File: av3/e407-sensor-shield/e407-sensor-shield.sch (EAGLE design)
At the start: 26 parts, among them CON1 CON1, CON2 CON1, CON4 CON4, J1 ROCKETBUS

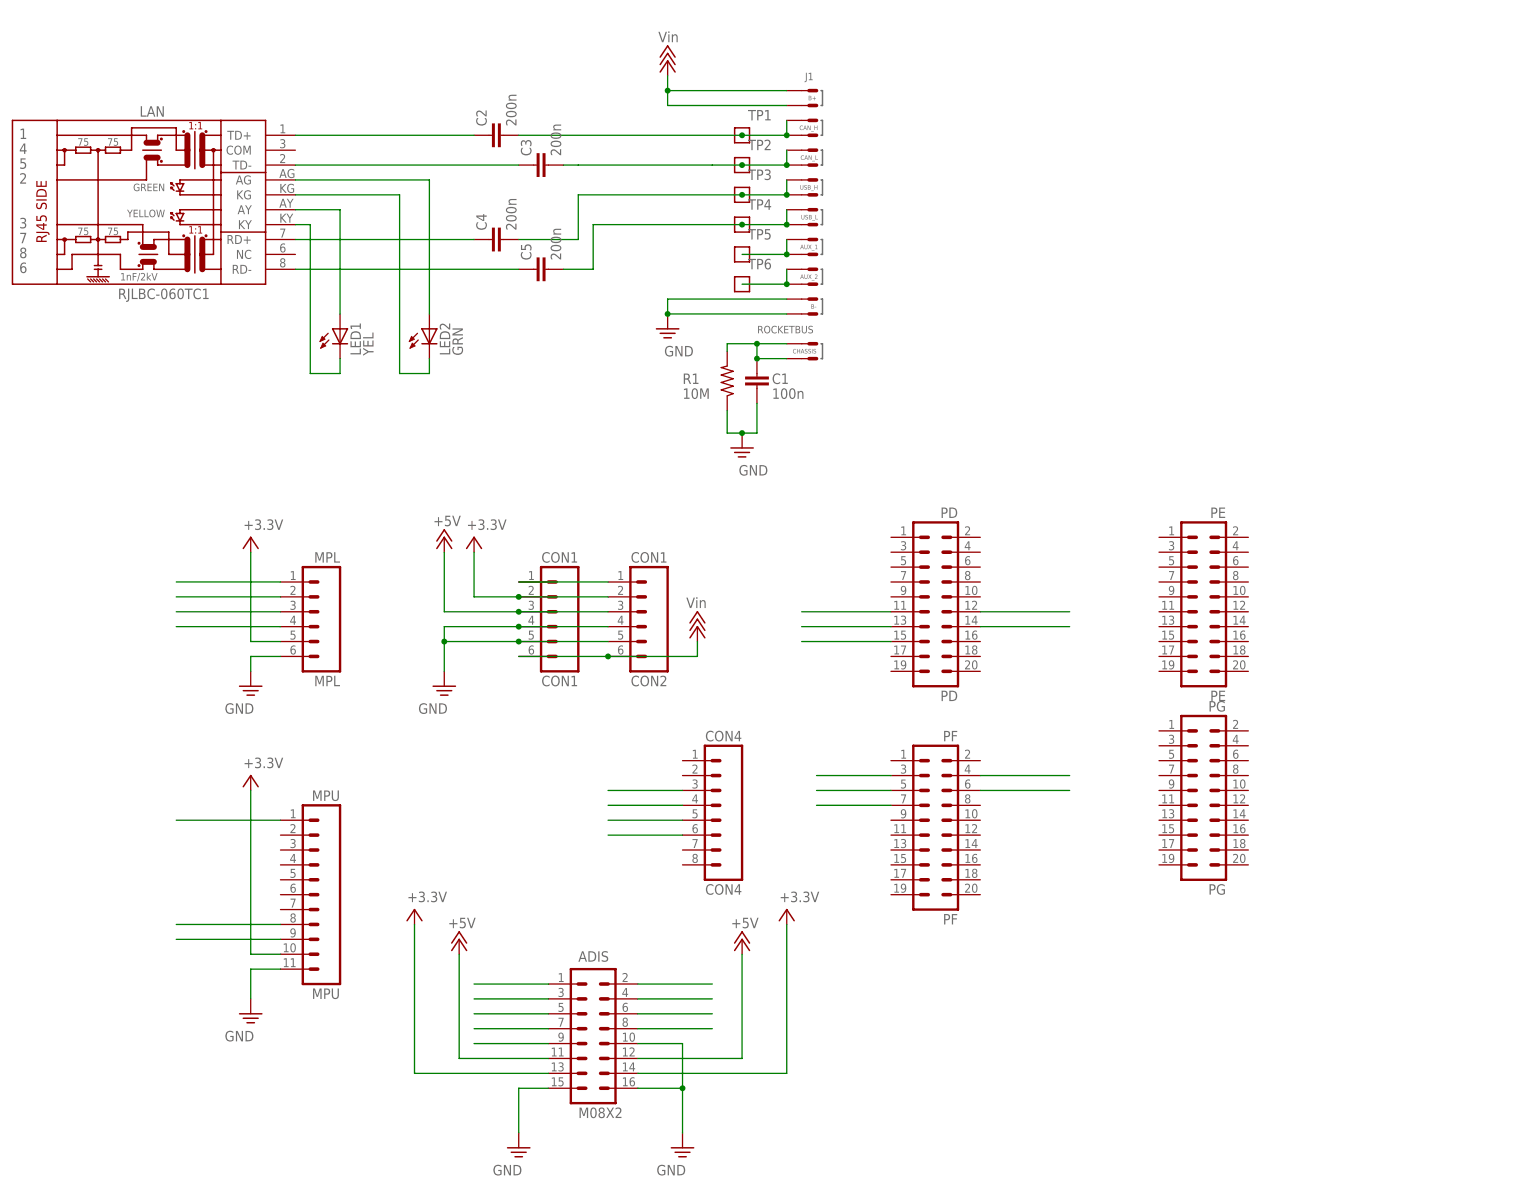
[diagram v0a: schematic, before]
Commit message: Added stupid EAGLE temporary files to the gitignore. Updated IMU adapter with sane net names so we could easily trace nets. And updated the e407 shield to add a RGB LED, correct some schematic mistakes found out while double checking connections, and updated to being routable on a PCB router.
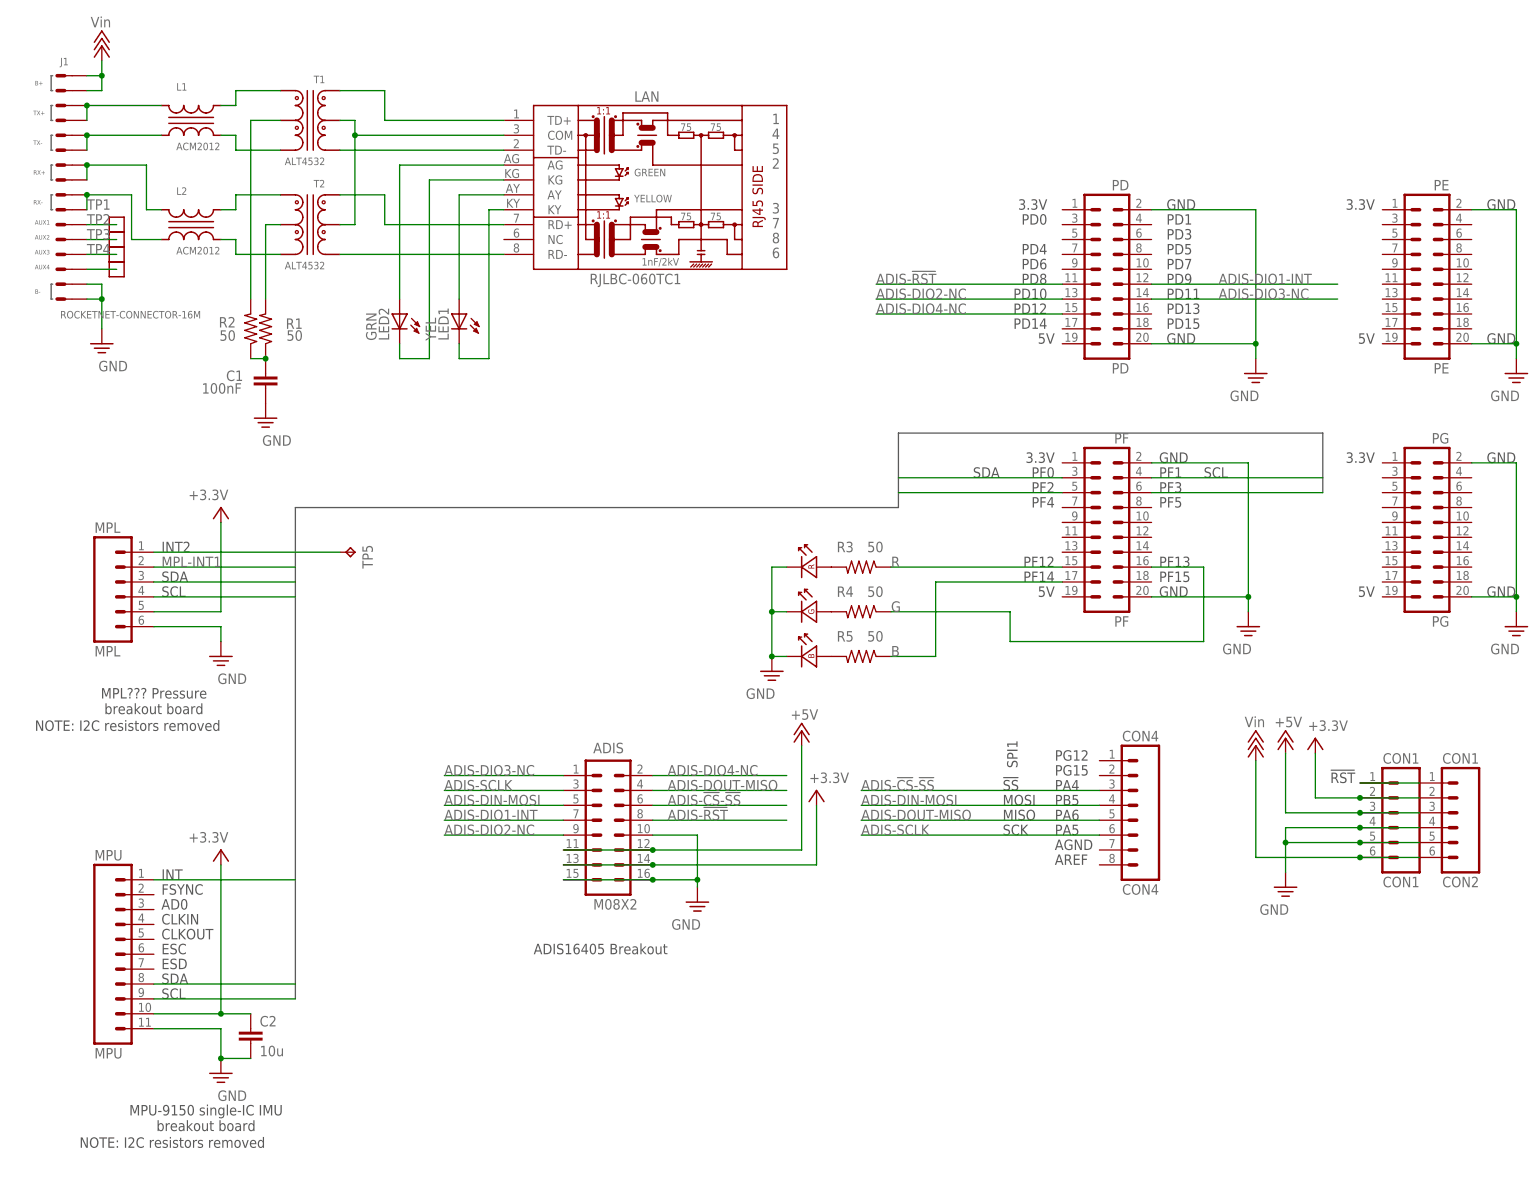
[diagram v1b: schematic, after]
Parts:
- removed C3, C4, C5: 200n, rcl_custom:C-EU0603-B-NOSILK
- removed TP6: TEST-POINT, apdm:TEST-POINT
- added L1, L2: ACM2012, magnetics:ACM2012
- added LED3: (no value), Tova:LED_RGB_PLCC-6
- added R2, R3, R4, R5: 50, rcl_custom:R-US_0603-B-NOSILK
- added T1, T2: ALT4532, magnetics:ALT4532
- C1: value 100n -> 100nF
- C2: value 200n -> 10u; device rcl_custom:C-EU0603-B-NOSILK -> rcl_custom:C-EU0805-B-NOSILK
- J1: value ROCKETBUS -> ROCKETNET-CONNECTOR-16M; device rocketbus:ROCKETBUS -> rocketnet-connector:ROCKETNET-CONNECTOR-16M
- R1: value 10M -> 50
- TP5: value TEST-POINT -> TPPAD1-13; device apdm:TEST-POINT -> testpad:TPPAD1-13
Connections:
- net C4D11 renamed ADIS-DIN-MOSI
- net C4D12 renamed ADIS-DOUT-MISO
- net PDP11 renamed ADIS-!RST
- net PDP12 renamed ADIS-DIO1-INT
- net PDP13 renamed ADIS-DIO2-NC
- net PDP14 renamed ADIS-DIO3-NC
- net PDP15 renamed ADIS-DIO4-NC
- net PFP06 renamed MPL-INT1
- removed net C4D10: ADIS.3, CON4.3
- removed net C4D13: ADIS.6, CON4.6
- new net ADIS-!CS!-!SS: ADIS.6, CON4.3
- new net ADIS-SCLK: ADIS.3, CON4.6
- new net B: PF.17, R5.1
- new net G: PF.16, R4.1
- new net N$19: J1.RX-@1, J1.RX-@2, L2.2
- new net N$20: J1.AUX4, TP4.1
- new net N$21: J1.AUX3, TP3.1
- new net N$22: J1.AUX2, TP2.1
- new net N$23: J1.AUX1, TP1.1
- new net N$24: LAN.COM, T1.6, T2.6
- new net N$25: C1.1, R1.1, R2.1
- new net N$26: R1.2, T2.3
- new net N$27: R2.2, T1.3
- new net N$28: LED3R.A, R3.2
- new net N$29: LED3G.A, R4.2
- new net N$30: LED3B.A, R5.2
- new net R: PF.15, R3.1
- net N$10: now also J1.RX+@1, J1.RX+@2, L2.1; no longer J1.AUX_2@1, J1.AUX_2@2, TP6.1
- net N$11: now also T1.1; no longer C2.1
- net N$12: now also T1.2; no longer C3.1
- net N$13: now also T2.1; no longer C4.1
- net N$14: now also T2.2; no longer C5.1
- net N$3: now also L1.4, T1.5; no longer C2.2, J1.CAN_H@1, J1.CAN_H@2, TP1.1
- net N$5: now also L1.3, T1.4; no longer C1.1, J1.CHASSIS@1, J1.CHASSIS@2, R1.2
- net N$6: now also L2.4, T2.5; no longer C3.2, J1.CAN_L@1, J1.CAN_L@2, TP2.1
- net N$7: now also L2.3, T2.4; no longer C4.2, J1.USB_H@1, J1.USB_H@2, TP3.1
- net N$8: now also J1.TX+@1, J1.TX+@2, L1.1; no longer C5.2, J1.USB_L@1, J1.USB_L@2, TP4.1
- net N$9: now also J1.TX-@1, J1.TX-@2, L1.2; no longer J1.AUX_1@1, J1.AUX_1@2, TP5.1
- net PFP07: now also TP5.TP; no longer PF.7
- net TRIPLE_BAR_GND: now also C2.2, LED3B.K, LED3G.K, LED3R.K, PD.2, PD.20, PE.2, PE.20, PF.2, PF.20, PG.2, PG.20; no longer R1.1
- net UP_ARROW: now also C2.1
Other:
- note added: "!RST"
- note added: "!SS"
- note added: "3.3V"
- note added: "5V"
- note added: "AD0"
- note added: "ADIS16405 Breakout"
- note added: "AGND"
- note added: "AREF"
- note added: "CLKIN"
- note added: "CLKOUT"
- note added: "ESC"
- note added: "ESD"
- note added: "FSYNC"
- note added: "GND"
- note added: "INT"
- note added: "INT2"
- note added: "MISO"
- note added: "MOSI"
- note added: "MPL??? Pressure breakout board"
- note added: "MPU-9150 single-IC IMU breakout board"
- note added: "NOTE: I2C resistors removed"
- note added: "PA4"
- note added: "PA5"
- note added: "PA6"
- note added: "PB5"
- note added: "PD0"
- note added: "PD1"
- note added: "PD10"
- note added: "PD11"
- note added: "PD12"
- note added: "PD13"
- note added: "PD14"
- note added: "PD15"
- note added: "PD3"
- note added: "PD4"
- note added: "PD5"
- note added: "PD6"
- note added: "PD7"
- note added: "PD8"
- note added: "PD9"
- note added: "PF0"
- note added: "PF1"
- note added: "PF12"
- note added: "PF13"
- note added: "PF14"
- note added: "PF15"
- note added: "PF2"
- note added: "PF3"
- note added: "PF4"
- note added: "PF5"
- note added: "PG12"
- note added: "PG15"
- note added: "SCK"
- note added: "SCL"
- note added: "SDA"
- note added: "SPI1"
- note removed: "C4D10"
- note removed: "C4D11"
- note removed: "C4D12"
- note removed: "C4D13"
- note removed: "PDP11"
- note removed: "PDP12"
- note removed: "PDP13"
- note removed: "PDP14"
- note removed: "PDP15"
- note removed: "PFP07"
- moved on the sheet: ADIS, C1, C2, CON1, CON2, CON4, LAN, LED1, LED2, MPL, MPU, PD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
